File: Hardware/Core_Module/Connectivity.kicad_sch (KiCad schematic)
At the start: 23 parts, among them J201 Connector_Left, J202 Connector_Bottom, J203 Connector_Right

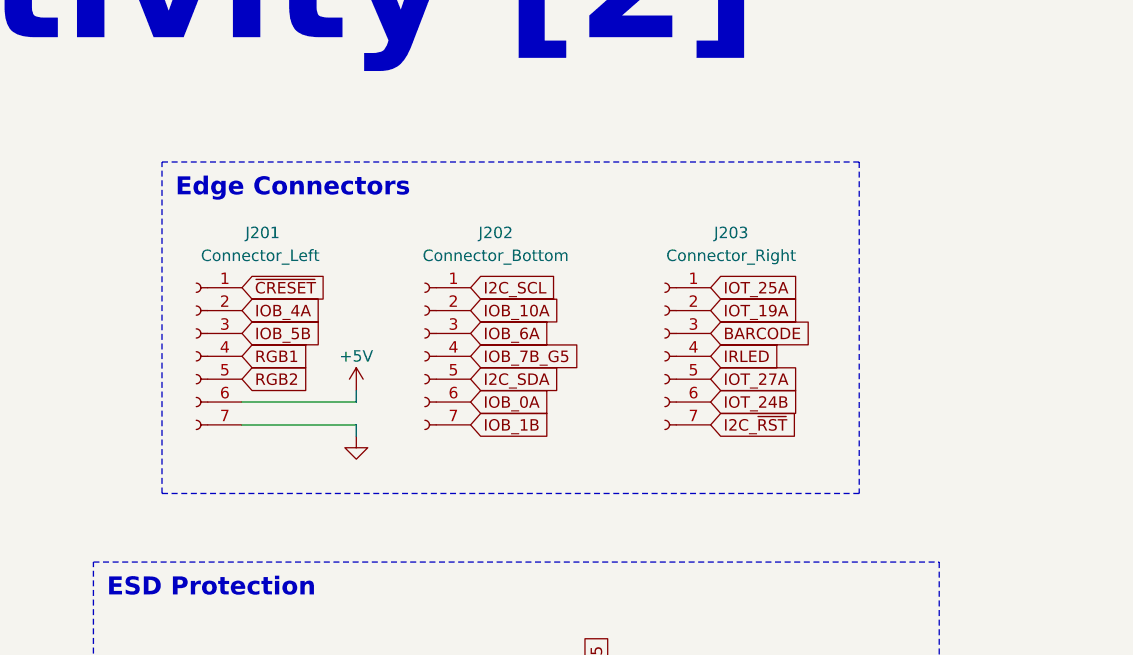
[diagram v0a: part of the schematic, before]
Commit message: Commit with restored changes after KiCad crash
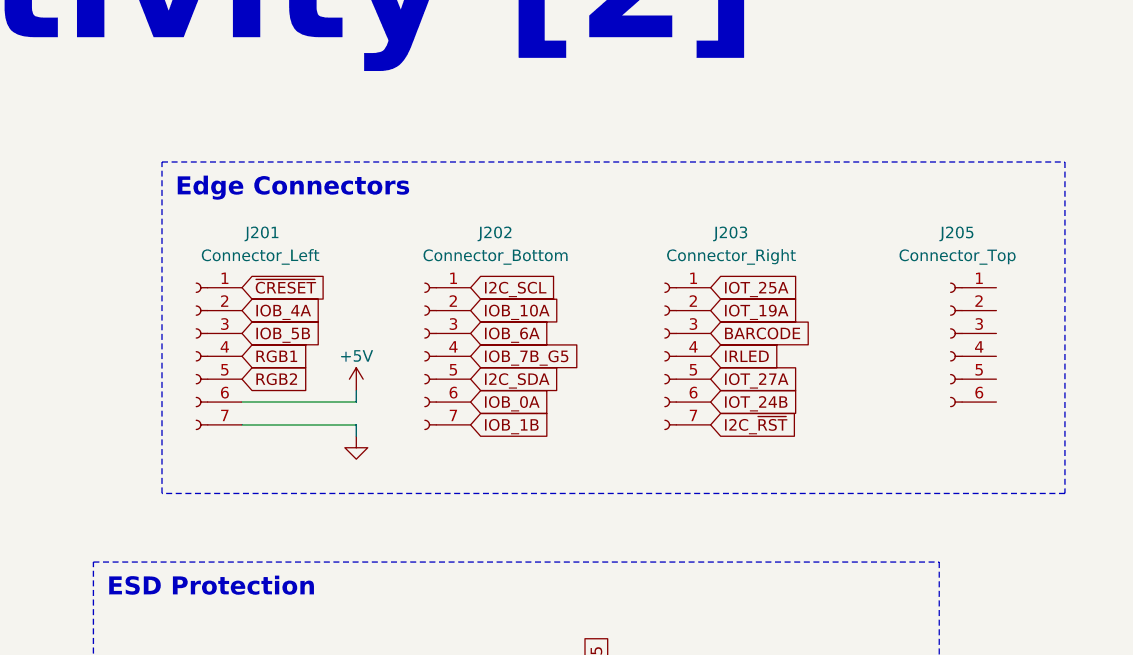
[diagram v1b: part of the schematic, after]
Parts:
- added J205: Connector_Top, Custom_VoxLink_Footprints:6-Pin_Casselated_Edge, symbol Connector:Conn_01x06_Socket
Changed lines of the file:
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@@
 		(exclude_from_sim no)
 		(at 106.68 46.99 0)
-		(size 77.47 36.83)
+		(size 100.33 36.83)
 		(margins 1.5 1.5 1.5 1.5)
 		(stroke
@@
 					(unit 1)
 				)
+			)
+		)
+	)
+	(symbol
+		(lib_id "Connector:Conn_01x06_Socket")
+		(at 194.31 66.04 0)
+		(mirror y)
+		(unit 1)
+		(body_style 1)
+		(exclude_from_sim no)
+		(in_bom yes)
+		(on_board yes)
+		(in_pos_files yes)
+		(dnp no)
+		(property "Reference" "J205"
+			(at 195.072 54.864 0)
+			(show_name no)
+			(do_not_autoplace no)
+			(effects
+				(font
+					(size 1.27 1.27)
+				)
+			)
+		)
+		(property "Value" "Connector_Top"
+			(at 195.072 57.404 0)
+			(show_name no)
+			(do_not_autoplace no)
+			(effects
+				(font
+					(size 1.27 1.27)
+				)
+			)
+		)
+		(property "Footprint" "Custom_VoxLink_Footprints:6-Pin_Casselated_Edge"
+			(at 194.31 66.04 0)
+			(hide yes)
+			(show_name no)
+			(do_not_autoplace no)
+			(effects
+				(font
+					(size 1.27 1.27)
+				)
+			)
+		)
+		(property "Datasheet" ""
+			(at 194.31 66.04 0)
+			(hide yes)
+			(show_name no)
+			(do_not_autoplace no)
+			(effects
+				(font
+					(size 1.27 1.27)
+				)
+			)
+		)
+		(property "Description" "Generic connector, single row, 01x06, script generated"
+			(at 194.31 66.04 0)
+			(hide yes)
+			(show_name no)
+			(do_not_autoplace no)
+			(effects
+				(font
+					(size 1.27 1.27)
+				)
+			)
+		)
+		(pin "3"
+		)
+		(pin "1"
+		)
+		(pin "4"
+		)
+		(pin "5"
+		)
+		(pin "2"
+		)
+		(pin "6"
+		)
+		(instances
+			(project "Core_Module"
+				(path "/398400c4-e3dc-429d-bda6-2a1ff309aedd/dbbe58bb-ba71-4ca5-8a9a-5dc2e79ec521"
+					(reference "J205")
+					(unit 1)
+				)

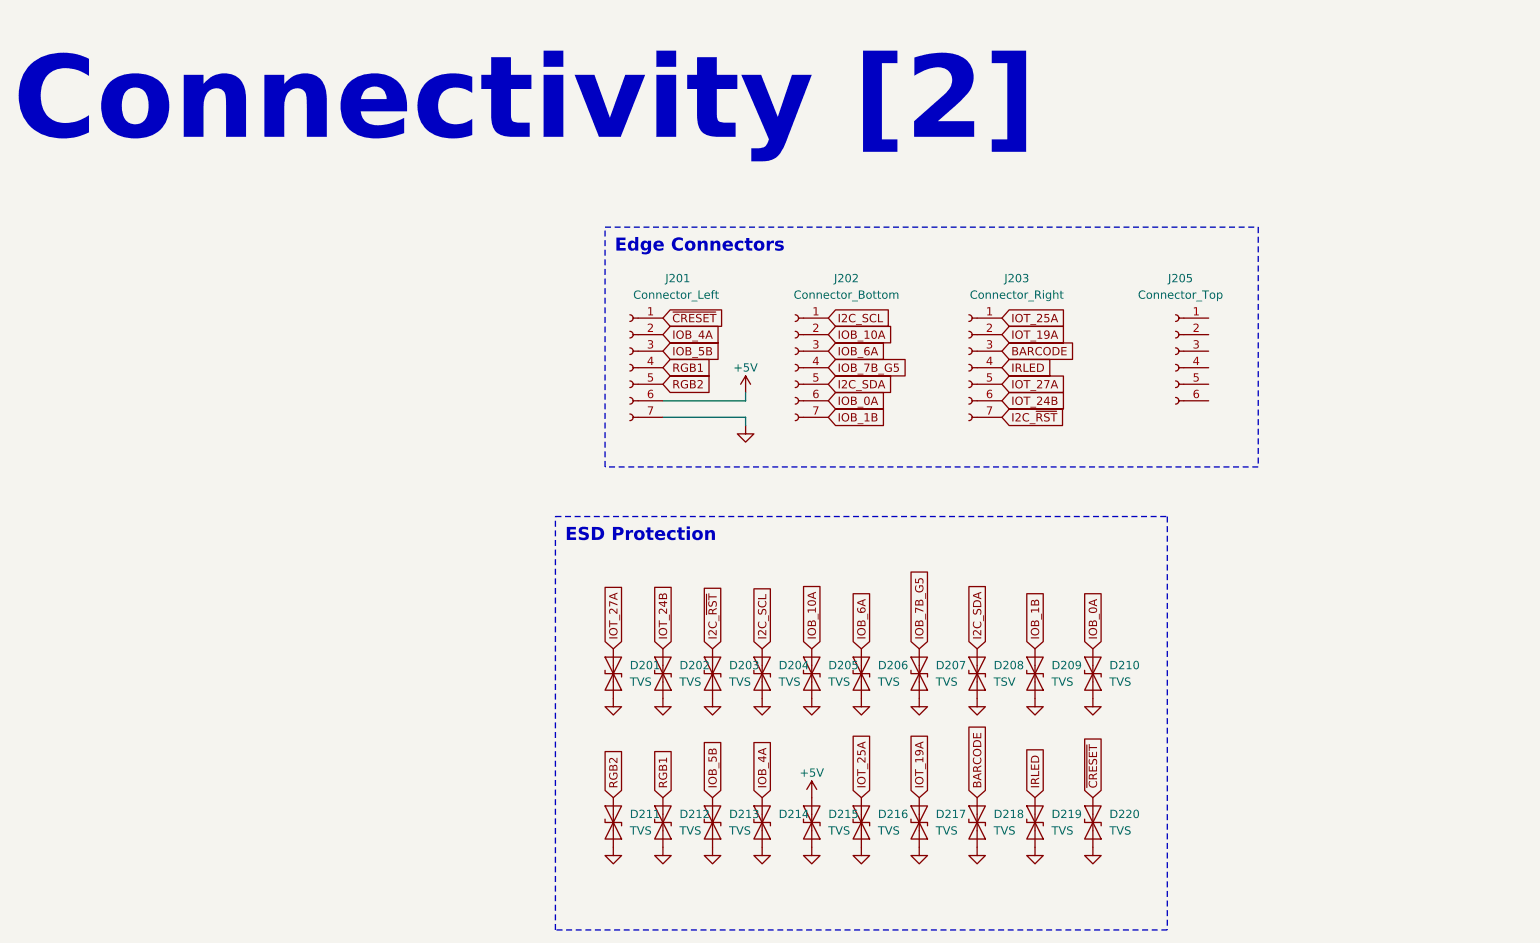
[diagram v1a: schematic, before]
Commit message: Finished Lattice Core, waiting for PCB Review
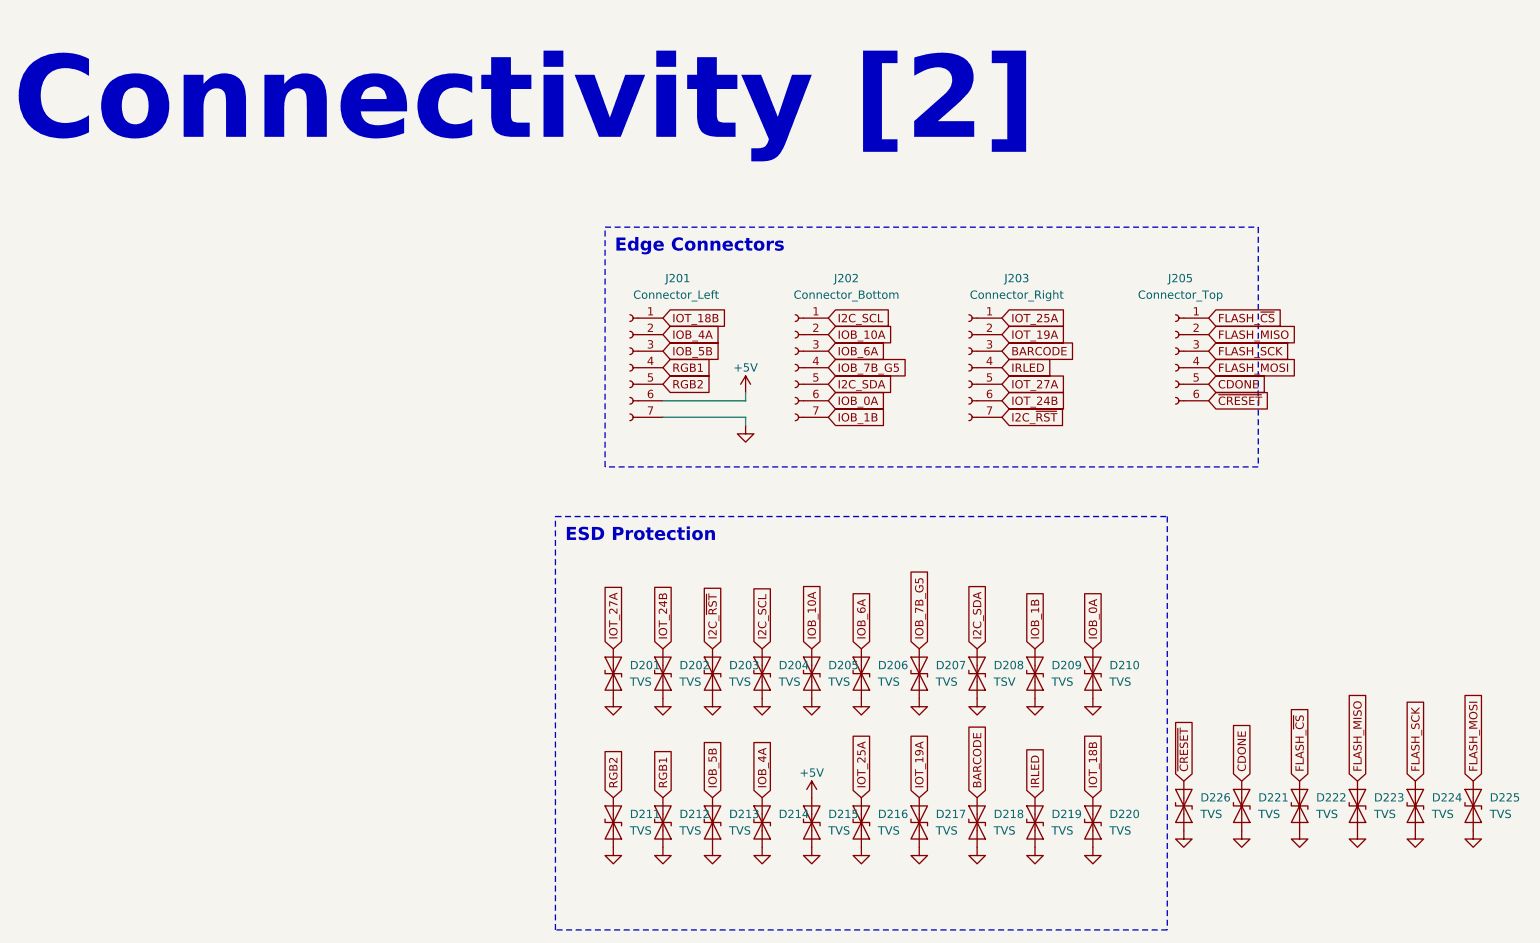
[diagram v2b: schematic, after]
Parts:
- added D221, D222, D223, D224, D225, D226: TVS, Custom_VoxLink_Footprints:WLL-2-3, symbol Diode:ESD9B3.3ST5G
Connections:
- net GND: now also D221.1 (A1), D222.1 (A1), D223.1 (A1), D224.1 (A1), D225.1 (A1), D226.1 (A1)
- net ~{CRESET}: now also J205.6 (Pin_6), D226.2 (A2); no longer D220.2 (A2), J201.1 (Pin_1)
- net FLASH_~{CS}: now reaches J205.1 (Pin_1)
- net FLASH_~{CS}: now also D222.2 (A2)
- net FLASH_MISO: now reaches J205.2 (Pin_2)
- net FLASH_MISO: now also D223.2 (A2)
- net FLASH_SCK: now reaches J205.3 (Pin_3)
- net FLASH_SCK: now also D224.2 (A2)
- net FLASH_MOSI: now reaches J205.4 (Pin_4)
- net FLASH_MOSI: now also D225.2 (A2)
- net CDONE: now reaches J205.5 (Pin_5)
- net CDONE: now also D221.2 (A2)
- new net IOT_18B: D220.2 (A2), J201.1 (Pin_1)

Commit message: Advanced Intel Core Module Development
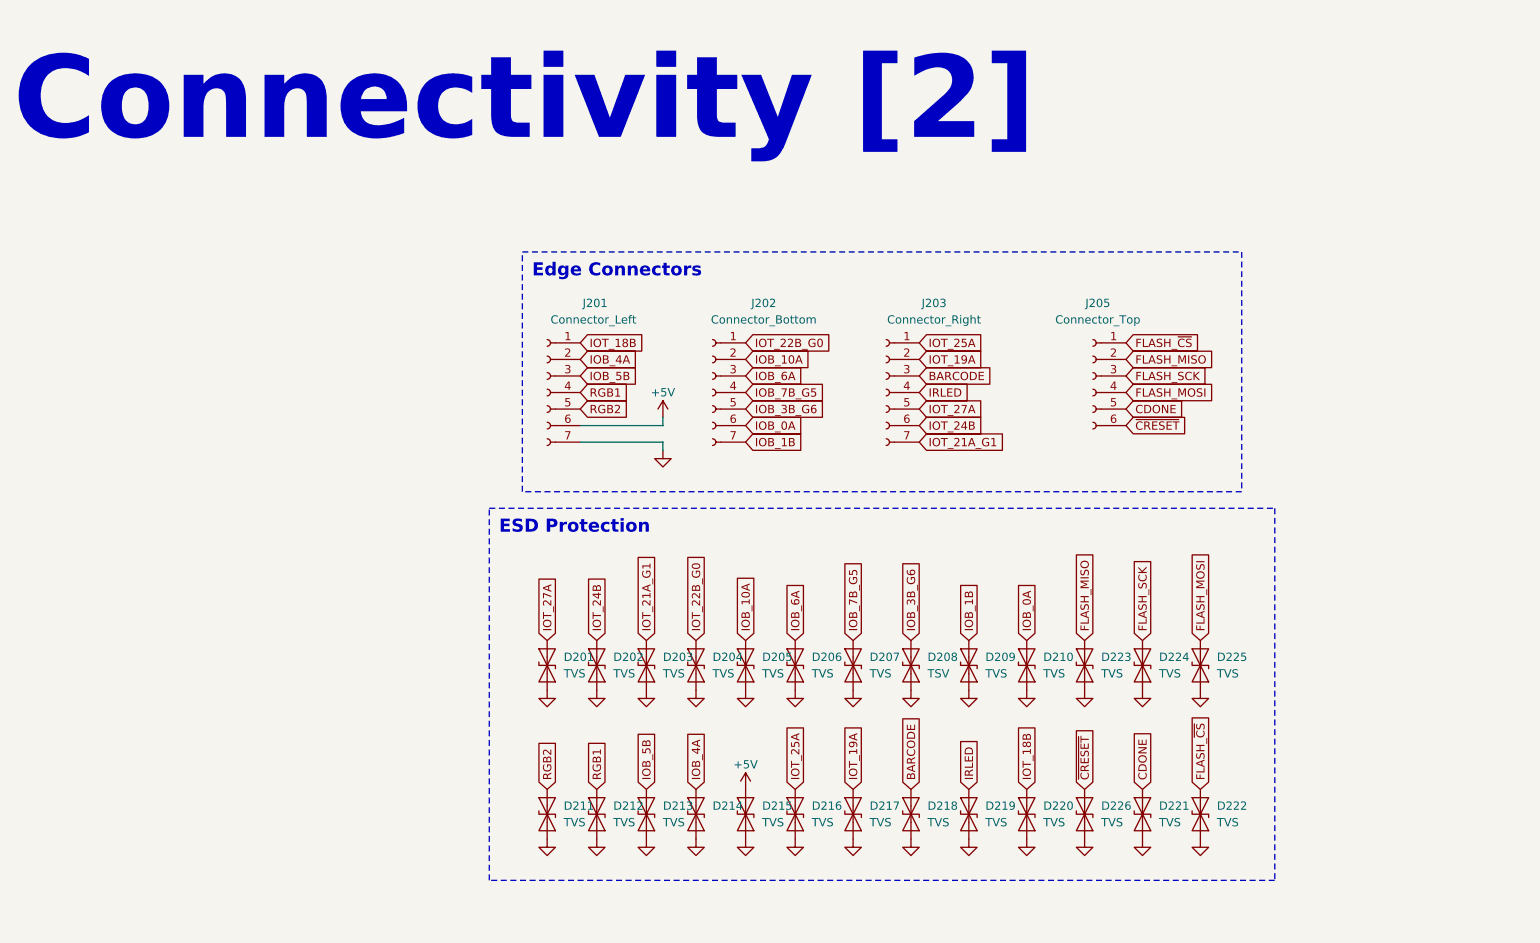
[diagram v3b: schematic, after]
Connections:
- net I2C_SCL renamed IOT_22B_G0
- net I2C_SDA renamed IOB_3B_G6
- net I2C_~{RST} renamed IOT_21A_G1
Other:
- moved on the sheet: D201, D202, D203, D204, D205, D206, D207, D208, D209, D210, D211, D212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
